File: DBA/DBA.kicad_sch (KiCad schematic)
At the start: 3 parts, among them U1 ESP32_NodeMCU_v1.1

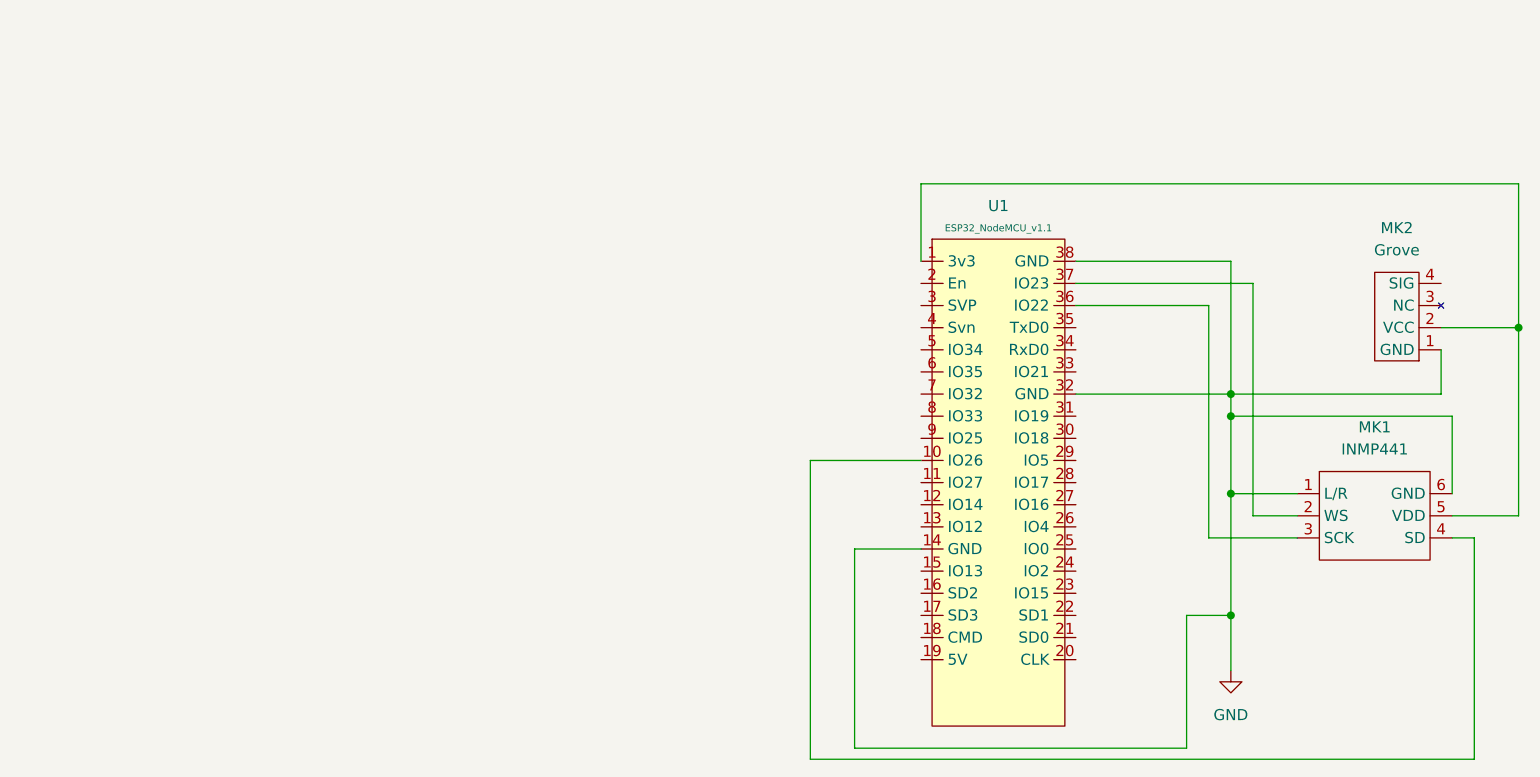
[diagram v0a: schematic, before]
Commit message: First complete model
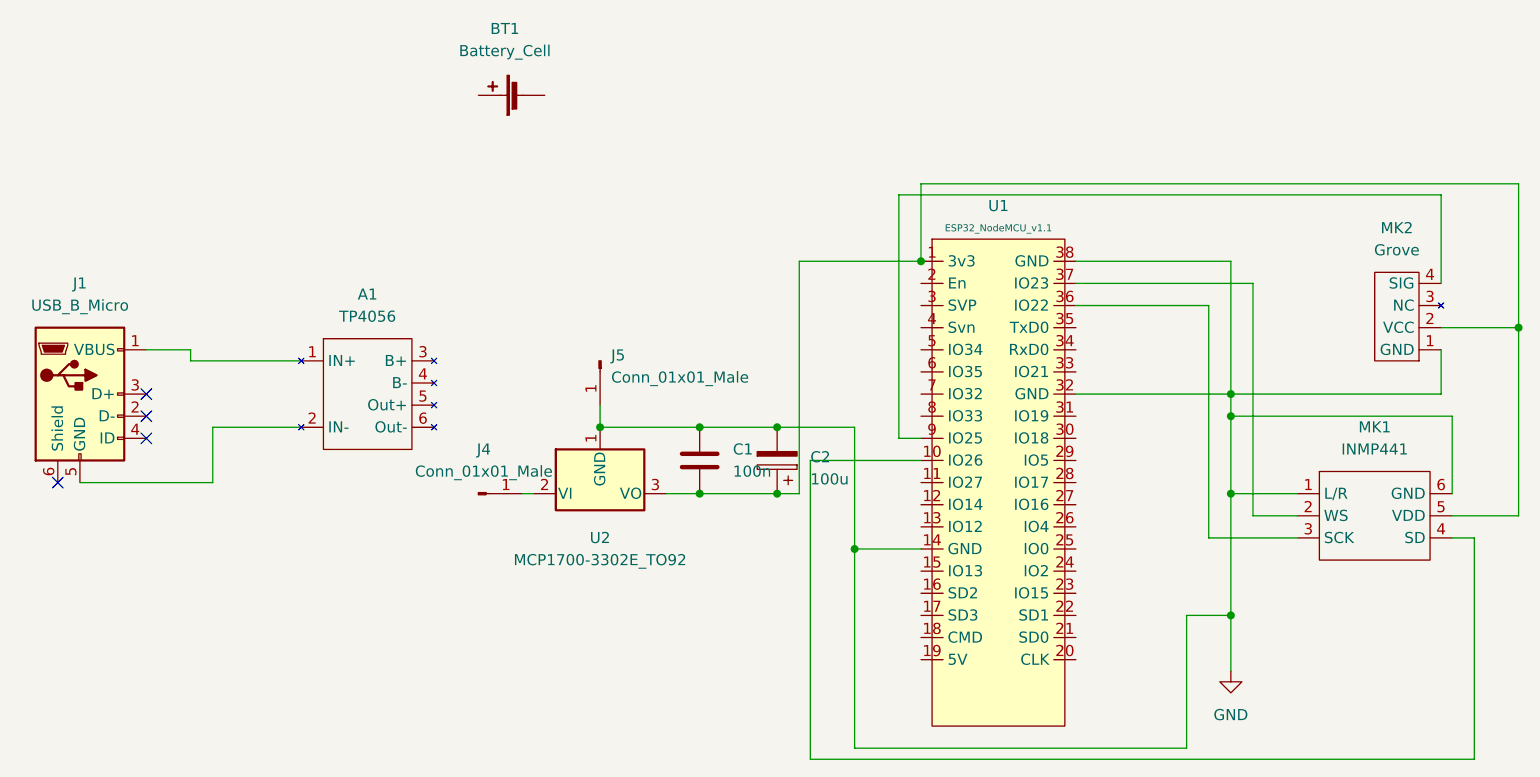
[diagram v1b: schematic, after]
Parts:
- added A1: TP4056, custom:TP4056Board, symbol Battery_Management:TP4056
- added BT1: Battery_Cell, Battery:BatteryHolder_Keystone_1042_1x18650, symbol Device:Battery_Cell
- added C1: 100n, Capacitor_THT:C_Radial_D6.3mm_H5.0mm_P2.50mm, symbol Device:C
- added C2: 100u, Capacitor_THT:CP_Radial_D5.0mm_P2.50mm, symbol Device:C_Polarized
- added J1: USB_B_Micro, symbol Connector:USB_B_Micro
- added J4, J5: Conn_01x01_Male, Connector_PinHeader_2.54mm:PinHeader_1x01_P2.54mm_Vertical, symbol Connector:Conn_01x01_Male
- added U2: MCP1700-3302E_TO92, Package_TO_SOT_THT:TO-92_Inline, symbol Regulator_Linear:MCP1700-3302E_TO92
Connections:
- net GND: now also C1.1, C2.2, J5.1 (Pin_1), U2.1 (GND)
- net at MK1.5 (VDD), MK2.2 (VCC), U1.1 (3v3): now also C1.2, C2.1, U2.3 (VO)
- net at U1.9 (IO25): now also MK2.4 (SIG)
- new net: J4.1 (Pin_1), U2.2 (VI)
- new net: A1.1 (IN+), J1.1 (VBUS)
- new net: A1.2 (IN-), J1.5 (GND)
- no-connect marks 0 -> 4
